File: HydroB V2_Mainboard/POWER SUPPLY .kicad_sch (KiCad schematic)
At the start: 27 parts, among them J1 Conn_01x02_Pin, J5 USB_C_Receptacle_USB2.0_16P, U3 TPS562200, U4 TPS54202DDC

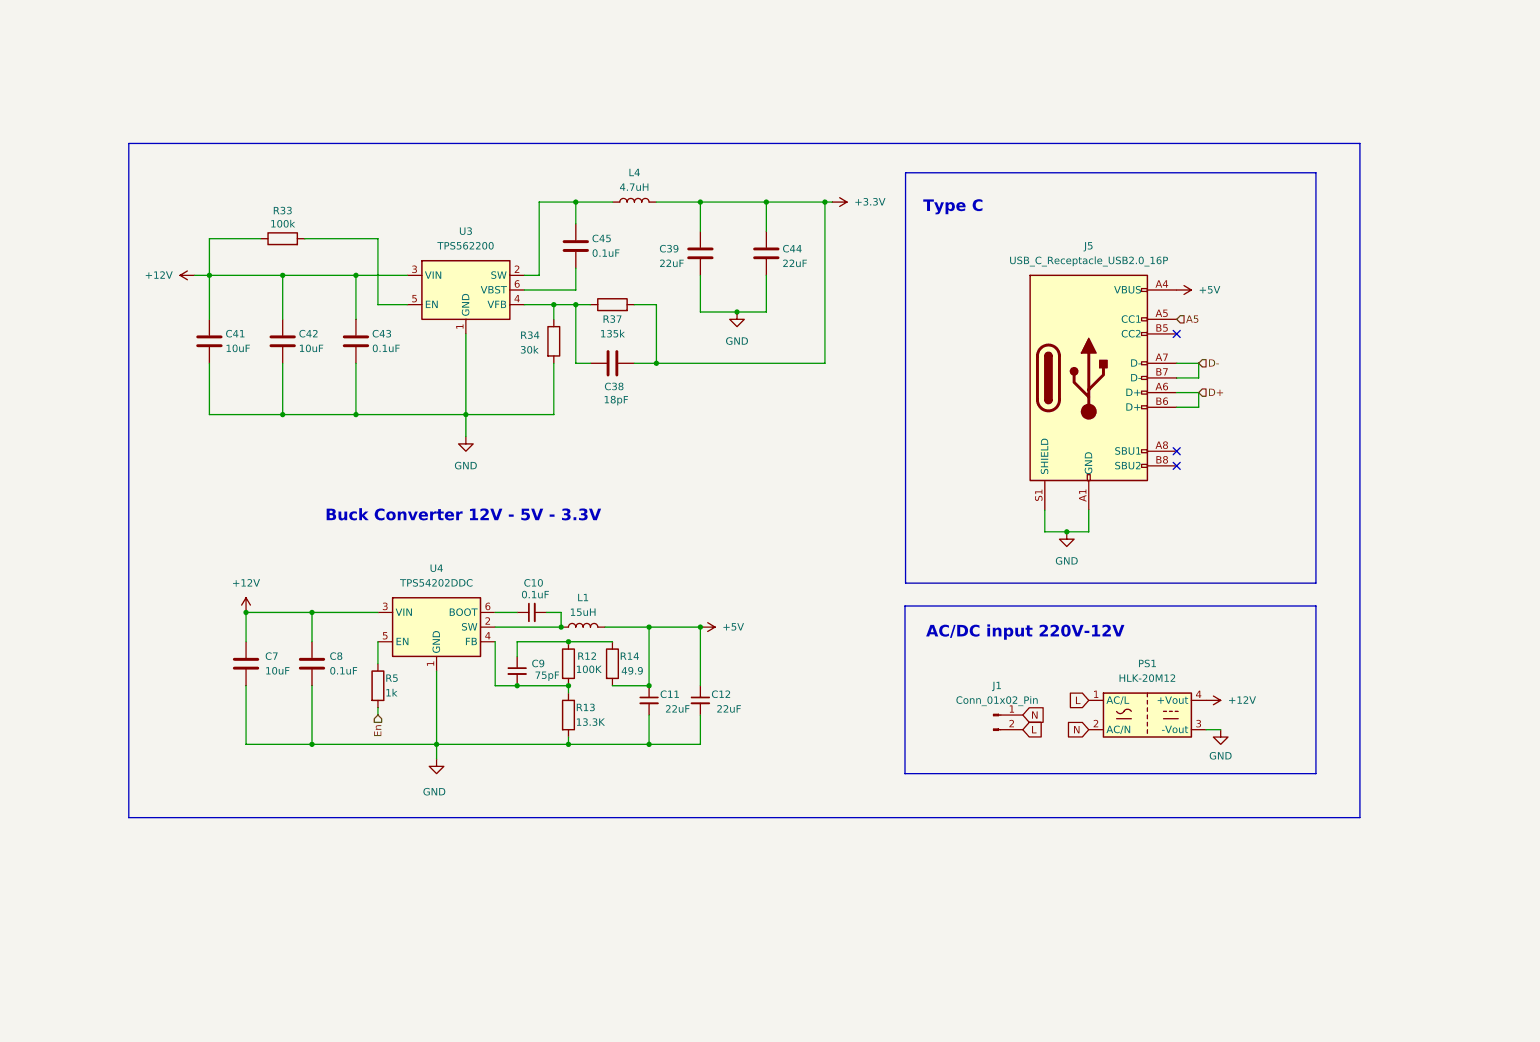
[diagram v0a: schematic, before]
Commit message: Mainboard schematic update
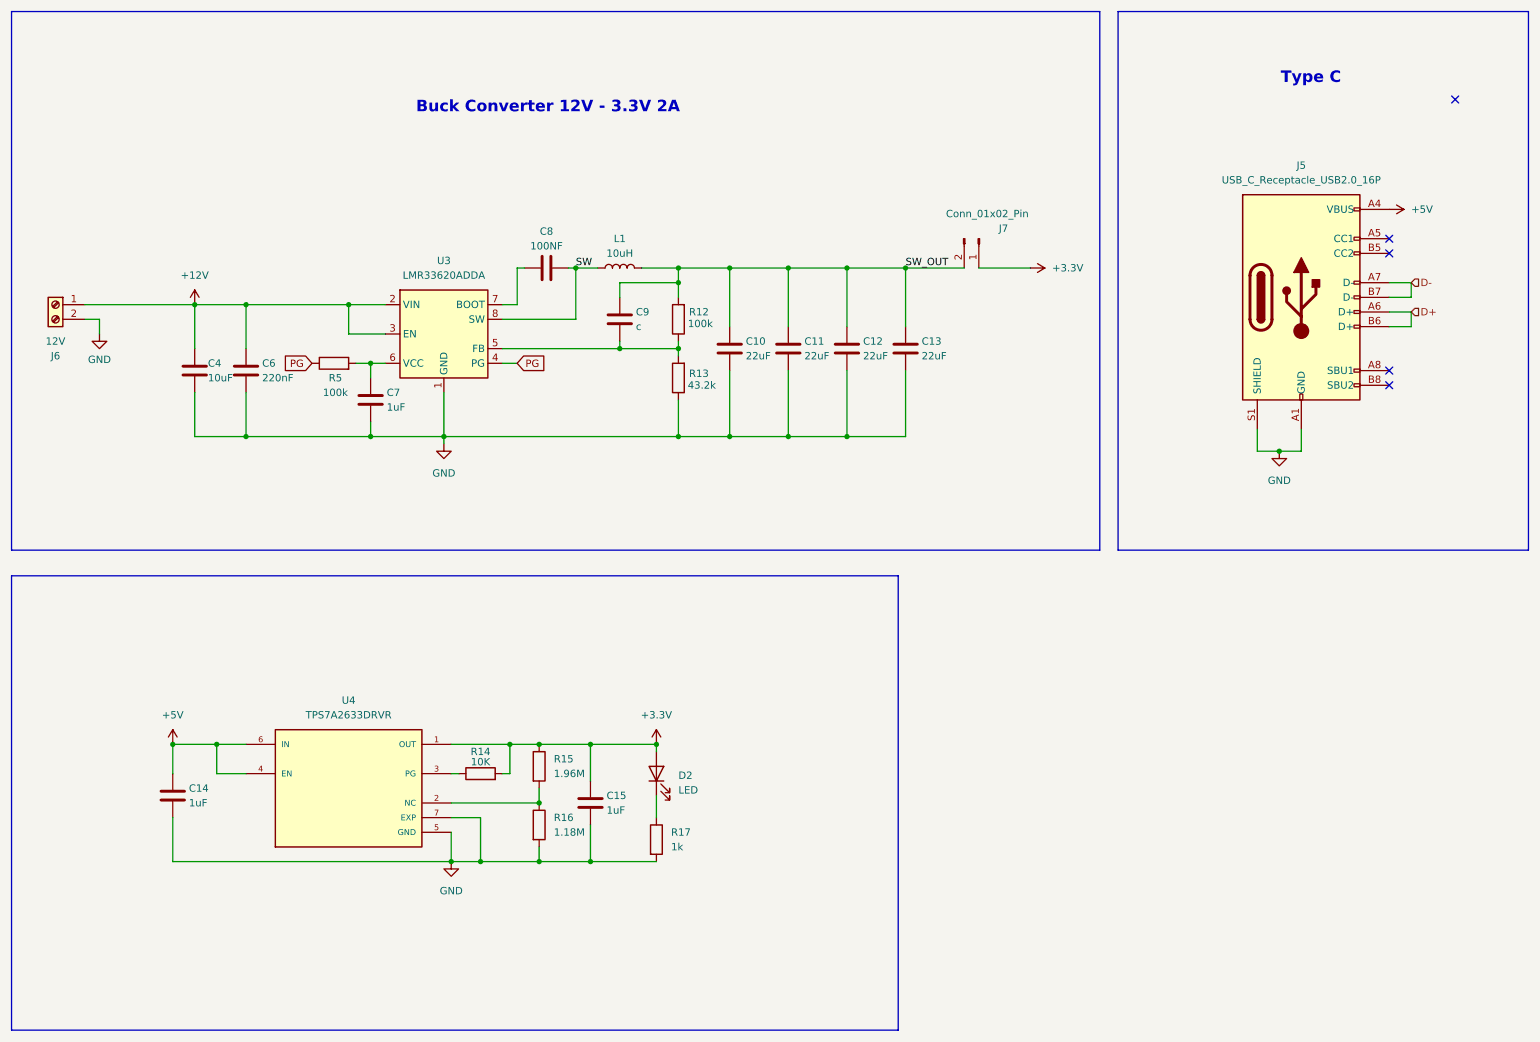
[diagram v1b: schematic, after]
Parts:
- removed C10: 0.1uF, Capacitor_SMD:C_0603_1608Metric, symbol Device:C_Small
- removed C11, C12: 22uF, Capacitor_SMD:C_0603_1608Metric, symbol Device:C_Small
- removed C38: 18pF, Capacitor_SMD:C_0603_1608Metric, symbol Device:C
- removed C39, C44: 22uF, Capacitor_SMD:C_0603_1608Metric, symbol Device:C
- removed C41: 10uF, Capacitor_SMD:CP_Elec_4x3, symbol Device:C
- removed C42: 10uF, Capacitor_SMD:C_0603_1608Metric, symbol Device:C
- removed C43, C45: 0.1uF, Capacitor_SMD:C_0603_1608Metric, symbol Device:C
- removed C9: 75pF, Capacitor_SMD:C_0603_1608Metric, symbol Device:C_Small
- removed J1: Conn_01x02_Pin, Connector_Phoenix_MC:PhoenixContact_MCV_1,5_2-G-3.81_1x02_P3.81mm_Vertical, symbol Connector:Conn_01x02_Pin
- removed L4: 4.7uH, Inductor_SMD:L_Bourns_SRP5030T, symbol Device:L
- removed PS1: HLK-20M12, Converter_ACDC:Converter_ACDC_Hi-Link_HLK-20Mxx, symbol Converter_ACDC:HLK-20M12
- removed R33: 100k, Resistor_SMD:R_0603_1608Metric, symbol Device:R
- removed R34: 30k, Resistor_SMD:R_0603_1608Metric, symbol Device:R
- removed R37: 135k, Resistor_SMD:R_0603_1608Metric, symbol Device:R
- removed U3: TPS562200, Package_TO_SOT_SMD:SOT-23-6, symbol Regulator_Switching:TPS562200
- removed U4: TPS54202DDC, Package_TO_SOT_SMD:SOT-23-6, symbol Regulator_Switching:TPS54202DDC
- added C10, C11, C12, C13: 22uF, Capacitor_SMD:C_0805_2012Metric, symbol Device:C
- added C14, C15: 1uF, Capacitor_SMD:C_0805_2012Metric, symbol Device:C
- added C4: 10uF, Capacitor_SMD:CP_Elec_4x3, symbol Device:C
- added C6: 220nF, Capacitor_SMD:C_0805_2012Metric, symbol Device:C
- added C9: c, Capacitor_SMD:C_0805_2012Metric, symbol Device:C
- added D2: LED, LED_SMD:LED_0603_1608Metric_Pad1.05x0.95mm_HandSolder, symbol Device:LED
- added J6: 12V, DC Conn:DC conn, symbol Connector:Screw_Terminal_01x02
- added J7: Conn_01x02_Pin, Connector_PinHeader_2.00mm:PinHeader_1x02_P2.00mm_Vertical, symbol Connector:Conn_01x02_Pin
- added R15: 1.96M, Resistor_SMD:R_0402_1005Metric, symbol Device:R
- added R16: 1.18M, Resistor_SMD:R_0402_1005Metric, symbol Device:R
- added R17: 1k, Resistor_SMD:R_0603_1608Metric, symbol Device:R
- added U3: LMR33620ADDA, Package_SO:Texas_HSOP-8-1EP_3.9x4.9mm_P1.27mm_ThermalVias, symbol Regulator_Switching:LMR33620ADDA
- added U4: TPS7A2633DRVR, TPS7A2633DRVR:SON65P200X200X80-7N, symbol TPS7A2633DRVR:TPS7A2633DRVR
- C7: value 10uF -> 1uF; footprint Capacitor_SMD:CP_Elec_4x3 -> Capacitor_SMD:C_0805_2012Metric
- C8: value 0.1uF -> 100NF
- L1: value 15uH -> 10uH; footprint Inductor_SMD:L_Vishay_IHLP-2020 -> Inductor_SMD:L_Bourns_SRP5030T
- R12: value 100K -> 100k
- R13: value 13.3K -> 43.2k
- R14: value 49.9 -> 10K
- R5: value 1k -> 100k; footprint Resistor_SMD:R_0402_1005Metric -> Resistor_SMD:R_0603_1608Metric
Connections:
- net +12V: now also C4.1, C6.1, J6.1 (Pin_1), U3.2 (VIN), U3.3 (EN); no longer C7.1, C8.1
- net +3.3V: now also R14.2, C15.1, D2.2 (A), J7.1 (Pin_1), R15.1, U4.1 (OUT)
- net +5V: now also C14.1, U4.4 (EN), U4.6 (IN); no longer L1.2, R14.2
- net GND: now also R13.1, C10.2, C11.2, C12.2, C13.2, C14.2, C15.2, C4.2, C6.2, J6.2 (Pin_2), R16.2, R17.2, U3.1 (GND), U3.9 (GND), U4.5 (GND), U4.7 (EXP); no longer C8.2, R13.2
- net SW_OUT: now reaches R12.2
- net SW_OUT: now also L1.2, C10.1, C11.1, C12.1, C13.1, C9.1, J7.2 (Pin_2); no longer R13.1
- net at R12.1: now also R13.2, C9.2, U3.5 (FB); no longer R14.1
- net PG: now reaches R5.1
- net PG: now also U3.4 (PG)
- net SW: now reaches L1.1
- net SW: now also C8.2, U3.8 (SW)
- net A5: no longer names the net of J5.A5 (CC1)
- net En: no longer names the net of R5.2
- net En: now also C7.1, U3.6 (VCC)
- new net: R15.2, R16.1, U4.2 (NC)
- new net: D2.1 (K), R17.1
- new net: R14.1, U4.3 (PG)
- new net: C8.1, U3.7 (BOOT)
- no-connect marks 3 -> 5
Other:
- note added: "Buck Converter 12V - 3.3V 2A"
- note removed: "AC/DC input 220V-12V"
- note removed: "Buck Converter 12V - 5V - 3.3V"
- moved on the sheet: J5
